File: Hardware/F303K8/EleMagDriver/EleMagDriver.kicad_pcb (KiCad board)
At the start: 2 copper layers, 114.3 x 76.2 mm, 49 parts, among them IC1 BD9E302EFJ-E2, IC2 TBD62083APG, IC3 TBD62083APG, IC4 TBD62083APG, J1 Jack-DC, J10 RelayD, J11 RelayE, J12 RelayF, J13 RelayG, J14 RelayH, J15 RelayI, J16 RelayJ, J17 Floppy_Power, J18 FloppyA, J19 Floppy_Power, J2 MotorDriverIn, J20 FloppyB, J21 Floppy_Power, J22 FloppyC, J3 MotorDriveOut, J4 SolenoidA, J5 SolenoidB, J6 StpMotor, J7 RelayA, J8 RelayB, J9 RelayC, U1 NUCLEO-F303K8

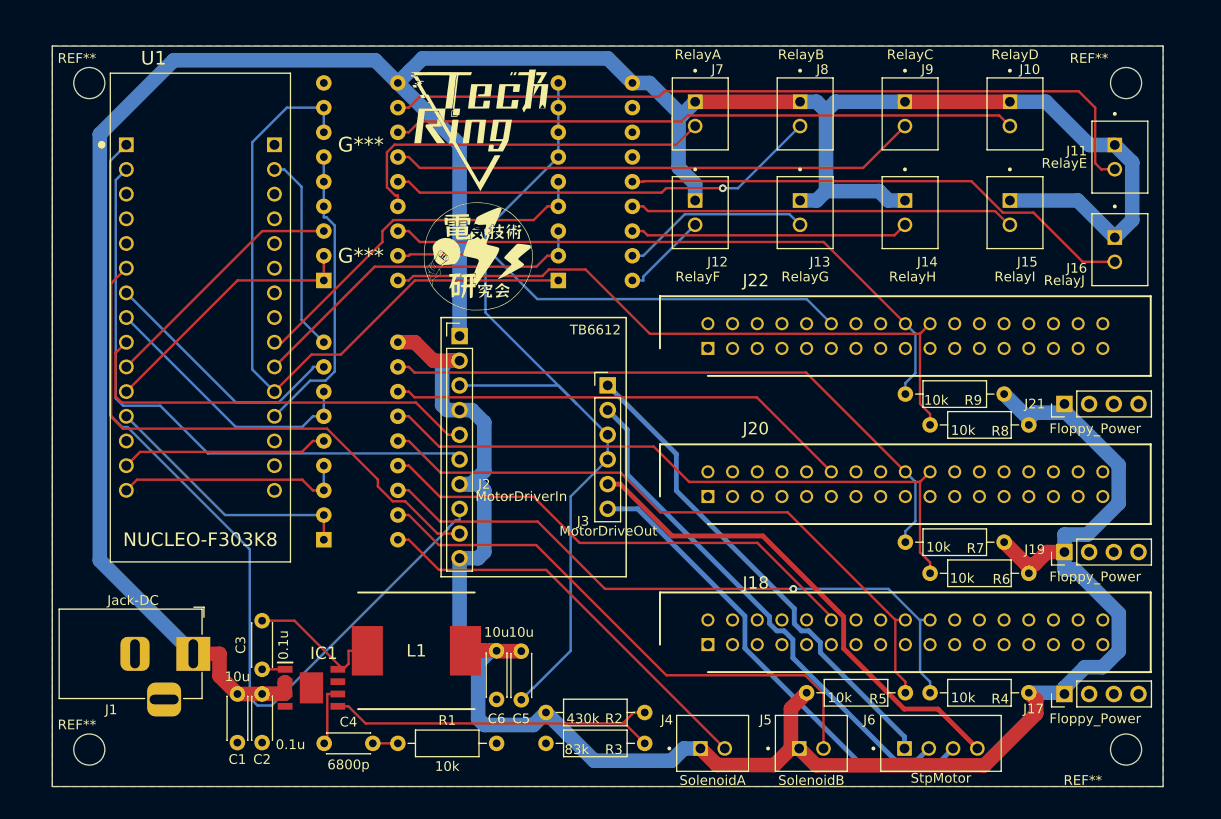
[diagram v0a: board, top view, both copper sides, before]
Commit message: substrate add guitar and more
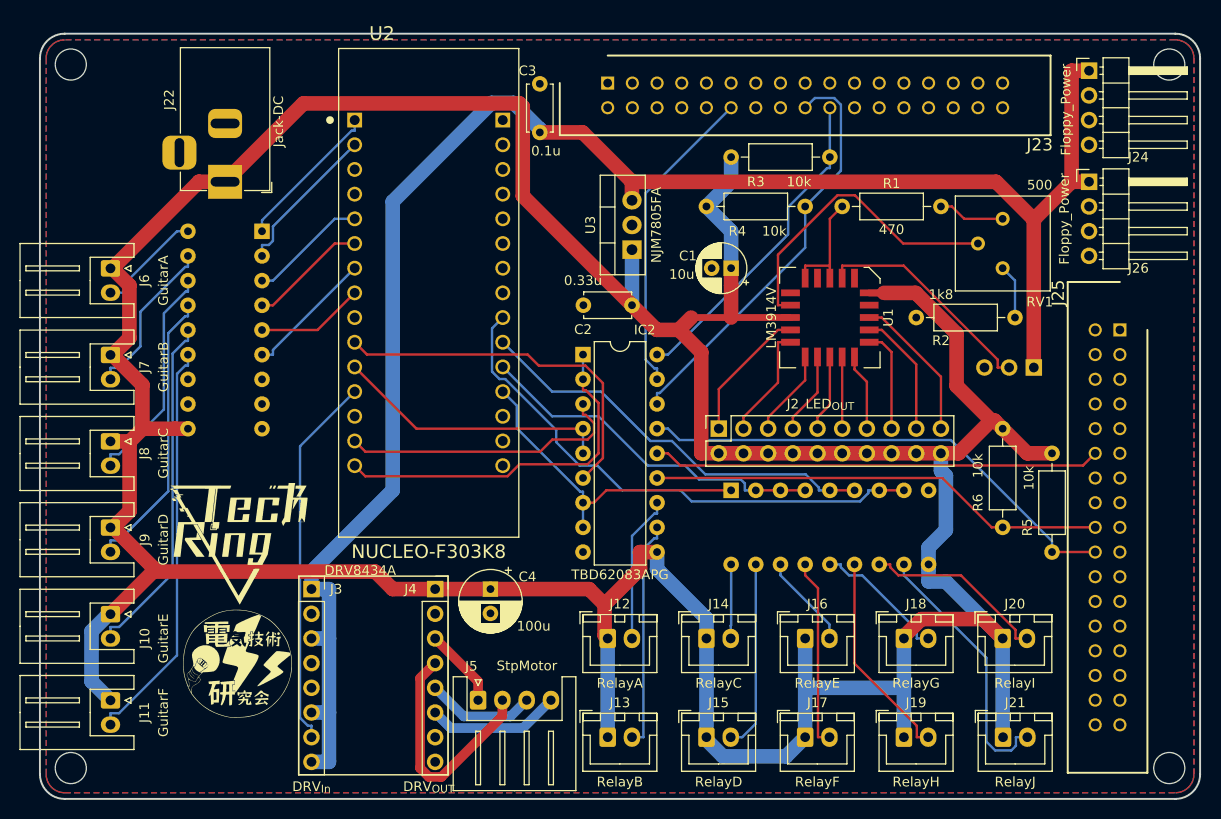
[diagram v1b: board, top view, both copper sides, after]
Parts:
- removed C5, C6: 10u, Capacitor_THT:C_Disc_D4.3mm_W1.9mm_P5.00mm
- removed IC4: TBD62083APG, Package_DIP:DIP-18_W7.62mm
- removed L1: 4.7u, INDPM120120X800N:INDPM120120X800N
- removed R7, R8, R9: 10k, Resistor_THT:R_Axial_DIN0207_L6.3mm_D2.5mm_P10.16mm_Horizontal
- removed the REF** at (105.4, 123.2)
- removed the REF** at (212.1, 54.6)
- removed the REF** at (212.1, 123.2)
- removed the REF** at (105.4, 54.6)
- added J23: FloppyA, Connector:SHDR34W70P254_2X17_5050X820X900P, F.Cu at (158.8, 54.6)
- added J24: Floppy_Power, Connector_PinHeader_2.54mm:PinHeader_1x04_P2.54mm_Horizontal, F.Cu at (208.3, 53.3)
- added J25: FloppyB, Connector:SHDR34W70P254_2X17_5050X820X900P, F.Cu at (211.5, 80.0)
- added J26: Floppy_Power, Connector_PinHeader_2.54mm:PinHeader_1x04_P2.54mm_Horizontal, F.Cu at (208.3, 64.8)
- added REF**: MountingHole_3.2mm_M3, MountingHole:MountingHole_3.2mm_M3, F.Cu at (216.5, 125.1)
- added REF**: MountingHole_3.2mm_M3, MountingHole:MountingHole_3.2mm_M3, F.Cu at (216.5, 52.7)
- added REF**: MountingHole_3.2mm_M3, MountingHole:MountingHole_3.2mm_M3, F.Cu at (103.5, 125.1)
- added REF**: MountingHole_3.2mm_M3, MountingHole:MountingHole_3.2mm_M3, F.Cu at (103.5, 52.7)
- added RV1: 500, Potentiometer_THT:Potentiometer_Bourns_3386P_Vertical, F.Cu at (199.4, 68.6)
- added U2: NUCLEO-F303K8, Module:MODULE_NUCLEO-F303K8, F.Cu at (140.3, 76.2)
- added U3: NJM7805FA, Package_TO_SOT_THT:TO-220-3_Vertical, F.Cu at (161.2, 71.8)
- C1: footprint Capacitor_THT:C_Disc_D4.3mm_W1.9mm_P5.00mm -> Capacitor_THT:CP_Radial_D5.0mm_P2.00mm
- C2: value 0.1u -> 0.33u; footprint Capacitor_THT:C_Disc_D4.3mm_W1.9mm_P5.00mm -> Capacitor_THT:C_Disc_D4.7mm_W2.5mm_P5.00mm
- C3: footprint Capacitor_THT:C_Disc_D4.3mm_W1.9mm_P5.00mm -> Capacitor_THT:C_Disc_D4.7mm_W2.5mm_P5.00mm
- C4: value 6800p -> 100u; footprint Capacitor_THT:C_Disc_D4.3mm_W1.9mm_P5.00mm -> Capacitor_THT:CP_Radial_D6.3mm_P2.50mm
- IC1: value BD9E302EFJ-E2 -> TBD62083APG; footprint SOIC127P600X100-9N:SOIC127P600X100-9N -> Package_DIP:DIP-18_W7.62mm; moved to B.Cu
- IC2: moved to F.Cu
- J1: value Jack-DC -> MIC_{IN}; footprint Connector_BarrelJack:BarrelJack_Horizontal -> Connector_PinSocket_2.54mm:PinSocket_1x03_P2.54mm_Vertical; moved to B.Cu
- J10: value RelayD -> GuitarE; footprint JST_B2B-XH-A(LF)(SN):JST_B2B-XH-A(LF)(SN) -> Connector_JST:JST_XH_S2B-XH-A_1x02_P2.50mm_Horizontal
- J11: value RelayE -> GuitarF; footprint JST_B2B-XH-A(LF)(SN):JST_B2B-XH-A(LF)(SN) -> Connector_JST:JST_XH_S2B-XH-A_1x02_P2.50mm_Horizontal
- J12: value RelayF -> RelayA; footprint JST_B2B-XH-A(LF)(SN):JST_B2B-XH-A(LF)(SN) -> Connector_JST:JST_XH_B2B-XH-A_1x02_P2.50mm_Vertical
- J13: value RelayG -> RelayB; footprint JST_B2B-XH-A(LF)(SN):JST_B2B-XH-A(LF)(SN) -> Connector_JST:JST_XH_B2B-XH-A_1x02_P2.50mm_Vertical
- J14: value RelayH -> RelayC; footprint JST_B2B-XH-A(LF)(SN):JST_B2B-XH-A(LF)(SN) -> Connector_JST:JST_XH_B2B-XH-A_1x02_P2.50mm_Vertical
- J15: value RelayI -> RelayD; footprint JST_B2B-XH-A(LF)(SN):JST_B2B-XH-A(LF)(SN) -> Connector_JST:JST_XH_B2B-XH-A_1x02_P2.50mm_Vertical
- J16: value RelayJ -> RelayE; footprint JST_B2B-XH-A(LF)(SN):JST_B2B-XH-A(LF)(SN) -> Connector_JST:JST_XH_B2B-XH-A_1x02_P2.50mm_Vertical
- J17: value Floppy_Power -> RelayF; footprint Connector_PinHeader_2.54mm:PinHeader_1x04_P2.54mm_Vertical -> Connector_JST:JST_XH_B2B-XH-A_1x02_P2.50mm_Vertical
- J18: value FloppyA -> RelayG; footprint SHDR34W70P254_2X17_5050X820X900P:SHDR34W70P254_2X17_5050X820X900P -> Connector_JST:JST_XH_B2B-XH-A_1x02_P2.50mm_Vertical
- J19: value Floppy_Power -> RelayH; footprint Connector_PinHeader_2.54mm:PinHeader_1x04_P2.54mm_Vertical -> Connector_JST:JST_XH_B2B-XH-A_1x02_P2.50mm_Vertical
- J2: value MotorDriverIn -> LED_{OUT}; footprint Connector_PinHeader_2.54mm:PinHeader_1x10_P2.54mm_Vertical -> Connector_PinSocket_2.54mm:PinSocket_2x10_P2.54mm_Vertical
- J20: value FloppyB -> RelayI; footprint SHDR34W70P254_2X17_5050X820X900P:SHDR34W70P254_2X17_5050X820X900P -> Connector_JST:JST_XH_B2B-XH-A_1x02_P2.50mm_Vertical
- J21: value Floppy_Power -> RelayJ; footprint Connector_PinHeader_2.54mm:PinHeader_1x04_P2.54mm_Vertical -> Connector_JST:JST_XH_B2B-XH-A_1x02_P2.50mm_Vertical
- J22: value FloppyC -> Jack-DC; footprint SHDR34W70P254_2X17_5050X820X900P:SHDR34W70P254_2X17_5050X820X900P -> Connector_BarrelJack:BarrelJack_Horizontal
- J3: value MotorDriveOut -> DRV_{In}; footprint Connector_PinHeader_2.54mm:PinHeader_1x06_P2.54mm_Vertical -> Connector_PinSocket_2.54mm:PinSocket_1x08_P2.54mm_Vertical
- J4: value SolenoidA -> DRV_{OUT}; footprint JST_B2B-XH-A(LF)(SN):JST_B2B-XH-A(LF)(SN) -> Connector_PinSocket_2.54mm:PinSocket_1x08_P2.54mm_Vertical
- J5: value SolenoidB -> StpMotor; footprint JST_B2B-XH-A(LF)(SN):JST_B2B-XH-A(LF)(SN) -> Connector_JST:JST_XH_S4B-XH-A_1x04_P2.50mm_Horizontal
- J6: value StpMotor -> GuitarA; footprint JST_B4B-XH-A(LF)(SN):JST_B4B-XH-A(LF)(SN) -> Connector_JST:JST_XH_S2B-XH-A_1x02_P2.50mm_Horizontal
- J7: value RelayA -> GuitarB; footprint JST_B2B-XH-A(LF)(SN):JST_B2B-XH-A(LF)(SN) -> Connector_JST:JST_XH_S2B-XH-A_1x02_P2.50mm_Horizontal
- J8: value RelayB -> GuitarC; footprint JST_B2B-XH-A(LF)(SN):JST_B2B-XH-A(LF)(SN) -> Connector_JST:JST_XH_S2B-XH-A_1x02_P2.50mm_Horizontal
- J9: value RelayC -> GuitarD; footprint JST_B2B-XH-A(LF)(SN):JST_B2B-XH-A(LF)(SN) -> Connector_JST:JST_XH_S2B-XH-A_1x02_P2.50mm_Horizontal
- R1: value 10k -> 470
- R2: value 430k -> 1k8
- R3: value 83k -> 10k
- U1: value NUCLEO-F303K8 -> LM3914V; footprint Nucleo-f303k8:MODULE_NUCLEO-F303K8 -> Package_LCC:PLCC-20
- moved J11 118.0 mm to (107.6, 118.1)
- moved J10 106.4 mm to (107.6, 109.3)
- moved J6 98.4 mm to (107.6, 73.7), turned to -90 degrees
- moved J9 92.6 mm to (107.6, 100.3)
- moved J1 91.4 mm to (202.6, 83.9), turned to 90 degrees
- moved J8 79.0 mm to (107.6, 91.5)
- moved R1 71.7 mm to (182.9, 67.3)
- moved J22 68.2 mm to (119.4, 64.8), turned to -90 degrees
- moved C1 67.1 mm to (171.4, 73.7), turned to 180 degrees
- moved J7 65.6 mm to (107.6, 82.6)
- moved U1 64.8 mm to (181.6, 78.7), turned to -90 degrees
- moved R2 63.1 mm to (200.7, 78.7), turned to 180 degrees
- moved J15 62.6 mm to (168.9, 121.9), turned to 0 degrees
- moved C3 62.2 mm to (151.8, 59.7)
- moved R3 61.0 mm to (171.4, 62.2), turned to 0 degrees
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- renumbered G*** to G0, G*** to G1
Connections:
- C3 pad 1: Net-(C3-Pad1) -> +5V
- C3 pad 2: Net-(C3-Pad2) -> GND
- C4 pad 1: Net-(C4-Pad1) -> +12V
- C4 pad 2: Net-(C4-Pad2) -> GND
- IC1 pad 1: Net-(C3-Pad1) -> /Guitar1
- IC1 pad 2: +12V -> /Guitar2
- IC1 pad 3: +12V -> /Guitar3
- IC1 pad 4: GND -> /Guitar4
- IC1 pad 5: Net-(IC1-Pad5) -> /Guitar5
- IC1 pad 6: Net-(C4-Pad1) -> /Guitar6
- IC1 pad 8: Net-(C3-Pad2) -> GND
- IC2 pad 1: /Solenoid -> /Step1
- IC2 pad 10: +5V -> +12V
- IC2 pad 11: Net-(IC2-Pad11) -> Net-(IC2-O8)
- IC2 pad 12: Net-(IC2-Pad12) -> Net-(IC2-O7)
- IC2 pad 13: Net-(IC2-Pad13) -> Net-(IC2-O6)
- IC2 pad 14: Net-(IC2-Pad14) -> Net-(IC2-O5)
- IC2 pad 15: Net-(IC2-Pad15) -> Net-(IC2-O4)
- IC2 pad 16: Net-(IC2-Pad16) -> Net-(IC2-O3)
- IC2 pad 17: Net-(IC2-Pad17) -> Net-(IC2-O2)
- IC2 pad 18: Net-(IC2-Pad18) -> Net-(IC2-O1)
- IC2 pad 2: /Solenoid -> /Step1
- IC2 pad 3: /Step1 -> /Direction1
- IC2 pad 4: /Step1 -> /Step2
- IC2 pad 5: /Direction1 -> /Step2
- IC2 pad 6: /Step2 -> /Direction2
- IC2 pad 7: /Step2 -> /Relay1
- IC2 pad 8: /Direction2 -> /Relay1
- IC3 pad 1: /Step3 -> /Relay1
- IC3 pad 11: Net-(J11-Pad2) -> Net-(IC3-O8)
- IC3 pad 12: Net-(J10-Pad2) -> Net-(IC3-O7)
- IC3 pad 13: Net-(IC3-Pad13) -> Net-(IC3-O6)
- IC3 pad 14: Net-(IC3-Pad14) -> Net-(IC3-O5)
- IC3 pad 15: Net-(IC3-Pad15) -> Net-(IC3-O4)
- IC3 pad 16: Net-(IC3-Pad16) -> Net-(IC3-O3)
- IC3 pad 17: Net-(IC3-Pad17) -> Net-(IC3-O2)
- IC3 pad 18: Net-(IC3-Pad18) -> Net-(IC3-O1)
- IC3 pad 2: /Step3 -> /Relay2
- IC3 pad 3: /Direction3 -> /Relay2
- IC3 pad 4: /Relay1 -> /Relay2
- IC3 pad 5: /Relay1 -> /Relay3
- IC3 pad 6: /Relay1 -> /Relay3
- IC3 pad 7: /Relay2 -> /Relay4
- IC3 pad 8: /Relay2 -> /Relay4
- J1 pad 1: +12V -> +5V
- J1 pad 2: GND -> Net-(J1-Pin_2)
- J1 pad 3: (no net) -> GND
- J10 pad 2: Net-(J10-Pad2) -> Net-(IC1-O5)
- J11 pad 2: Net-(J11-Pad2) -> Net-(IC1-O6)
- J12 pad 2: Net-(J12-Pad2) -> Net-(IC2-O7)
- J13 pad 2: Net-(J13-Pad2) -> Net-(IC2-O8)
- J14 pad 2: Net-(J14-Pad2) -> Net-(IC3-O1)
- J15 pad 2: Net-(J15-Pad2) -> Net-(IC3-O2)
- J16 pad 2: Net-(J16-Pad2) -> Net-(IC3-O3)
- J17 pad 1: +5V -> +12V
- J17 pad 2: GND -> Net-(IC3-O4)
- J18 pad 1: unconnected-(J18-Pad1) -> +12V
- J18 pad 2: unconnected-(J18-Pad2) -> Net-(IC3-O5)
- J19 pad 1: +5V -> +12V
- J19 pad 2: GND -> Net-(IC3-O6)
- J2 pad 1: +12V -> Net-(J2-Pin_1)
- J2 pad 10: +5V -> +12V
- J2 pad 2: +5V -> +12V
- J2 pad 3: GND -> Net-(J2-Pin_3)
- J2 pad 4: +5V -> +12V
- J2 pad 5: /Stp_BN -> Net-(J2-Pin_5)
- J2 pad 6: /Stp_B -> +12V
- J2 pad 7: +5V -> Net-(J2-Pin_7)
- J2 pad 8: /Stp_A -> +12V
- J2 pad 9: /Stp_AN -> Net-(J2-Pin_9)
- J20 pad 1: unconnected-(J20-Pad1) -> +12V
- J20 pad 2: unconnected-(J20-Pad2) -> Net-(IC3-O7)
- J21 pad 1: +5V -> +12V
- J21 pad 2: GND -> Net-(IC3-O8)
- J22 pad 1: unconnected-(J22-Pad1) -> +12V
- J22 pad 2: unconnected-(J22-Pad2) -> GND
- J22 pad 3: unconnected-(J22-Pad3) -> (no net)
- J3 pad 1: /Motor_OutAN -> +5V
- J3 pad 2: /Motor_OutA -> GND
- J3 pad 3: GND -> +5V
- J3 pad 4: GND -> unconnected-(J3-Pin_4-Pad4)
- J3 pad 5: /Motor_OutBN -> unconnected-(J3-Pin_5-Pad5)
- J3 pad 6: /Motor_OutB -> +5V
- J4 pad 1: +5V -> +12V
- J4 pad 2: Net-(IC2-Pad18) -> GND
- J5 pad 1: +5V -> /Motor_OutB
- J5 pad 2: Net-(IC2-Pad17) -> /Motor_OutBN
- J6 pad 1: /Motor_OutAN -> +12V
- J6 pad 2: /Motor_OutA -> Net-(IC1-O1)
- J7 pad 2: Net-(IC3-Pad15) -> Net-(IC1-O2)
- J8 pad 2: Net-(IC3-Pad14) -> Net-(IC1-O3)
- J9 pad 2: Net-(IC3-Pad13) -> Net-(IC1-O4)
- R1 pad 1: Net-(C4-Pad2) -> Net-(U1-REFOUT)
- R1 pad 2: GND -> Net-(R1-Pad2)
- R2 pad 1: +5V -> Net-(R2-Pad1)
- R2 pad 2: Net-(IC1-Pad5) -> GND
- R3 pad 1: Net-(IC1-Pad5) -> +12V
- R3 pad 2: GND -> Net-(IC2-O1)
- R4 pad 1: +5V -> +12V
- R4 pad 2: Net-(IC2-Pad16) -> Net-(IC2-O3)
- R5 pad 1: +5V -> +12V
- R5 pad 2: Net-(IC2-Pad14) -> Net-(IC2-O4)
- R6 pad 1: +5V -> +12V
- R6 pad 2: Net-(IC2-Pad13) -> Net-(IC2-O6)
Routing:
- net +12V: track 268.0 -> 431.6 mm
- net GND: track 108.8 -> 0.00 mm
- net /Stp_A: track 94.9 -> 0.00 mm
- net Net-(J11-Pad2): track 81.2 -> 0.00 mm
- net Net-(IC3-Pad18): track 68.2 -> 0.00 mm
- net Net-(IC2-Pad16): track 68.2 -> 0.00 mm, vias 1 -> 0
- net Net-(IC2-Pad13): track 67.8 -> 0.00 mm
- net Net-(IC2-Pad14): track 67.8 -> 0.00 mm
- net Net-(IC2-Pad11): track 64.8 -> 0.00 mm
- net Net-(IC3-Pad16): track 64.3 -> 0.00 mm
- net Net-(J10-Pad2): track 64.1 -> 0.00 mm
- net /Stp_B: track 62.0 -> 0.00 mm
- net /Stp_AN: track 57.2 -> 0.00 mm
- net Net-(IC2-Pad17): track 57.1 -> 0.00 mm
- net Net-(IC3-Pad13): track 54.4 -> 0.00 mm
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- added copper zone on B.Cu, net GND
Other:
- board size 114.3 x 76.2 mm -> 119.4 x 78.7 mm
- board text added: "DRV8434A"
- board text removed: "TB6612"
